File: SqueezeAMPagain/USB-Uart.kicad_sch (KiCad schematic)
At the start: 12 parts, among them J5 USB_B_Micro, J9 Conn_01x06_Pin, Q4 Q_NPN_BEC, Q5 Q_NPN_BEC, U3 CP2102N-Axx-xQFN28

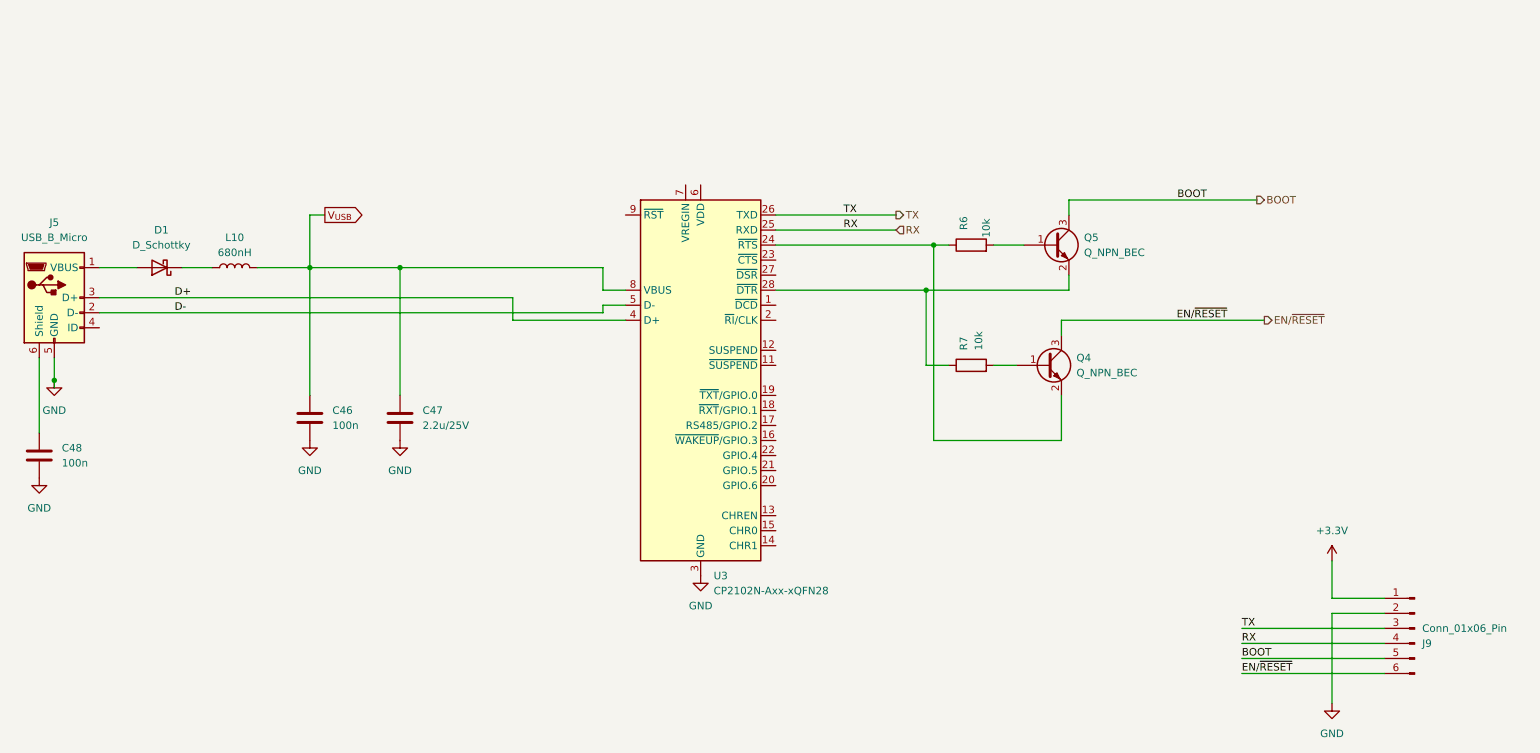
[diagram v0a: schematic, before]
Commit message: Update SqueezeAMPagain.kicad_pcb, SqueezeAMPagain.kicad_prl, USB-Uart.kicad_sch, and 4 more files
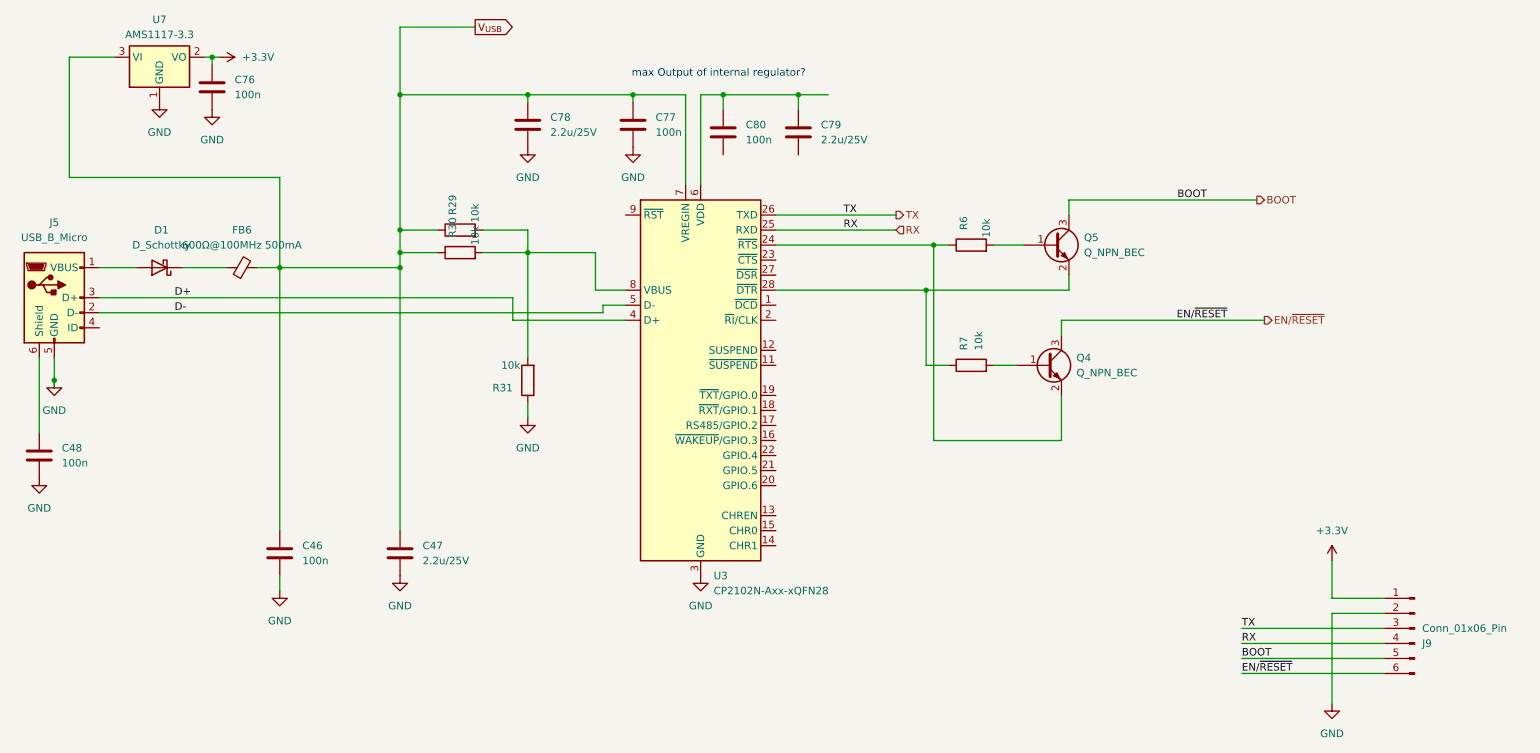
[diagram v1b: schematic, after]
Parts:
- removed L10: 680nH, Inductor_SMD:L_0805_2012Metric, symbol Device:L
- added C76, C77, C80: 100n, Capacitor_SMD:C_0603_1608Metric, symbol Device:C
- added C78, C79: 2.2u/25V, Capacitor_SMD:C_0805_2012Metric, symbol Device:C
- added FB6: 600Ω@100MHz 500mA, Inductor_SMD:L_0805_2012Metric, symbol Device:FerriteBead_Small
- added R29, R30, R31: 10k, Resistor_SMD:R_0603_1608Metric, symbol Device:R
- added U7: AMS1117-3.3, Package_TO_SOT_SMD:SOT-223-3_TabPin2, symbol Regulator_Linear:AMS1117-3.3
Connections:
- net +3.3V: now also C76.1, U7.2 (VO)
- net GND: now also C76.2, C77.2, C78.2, R31.1, U7.1 (GND)
- net V_{USB}: now also U3.7 (VREGIN), C77.1, C78.1, FB6.2, R29.1, R30.1, U7.3 (VI); no longer U3.8 (VBUS)
- net at D1.1 (K): now also FB6.1
- net at U3.6 (VDD): now also C79.1, C80.1
- new net: R29.2, R30.2, R31.2, U3.8 (VBUS)
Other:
- note added: "max Output of internal regulator?"
- moved on the sheet: C46, C47
